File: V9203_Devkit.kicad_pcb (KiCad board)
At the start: 2 copper layers, 50 x 50 mm, 101 parts, among them J1 RJ45, J10 GS3, J2 CONN_01X16, J3 CONN_01X12, J4 Screw_Terminal_1x04, J5 GROVE-CONNECTOR-SMD-90D(4+2P-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, J6 CONN_01X09, J7 GS3, J8 GS3, J9 CONN_01X06, U1 V9203, U2 ROF-78E, Y1 Crystal_GND24

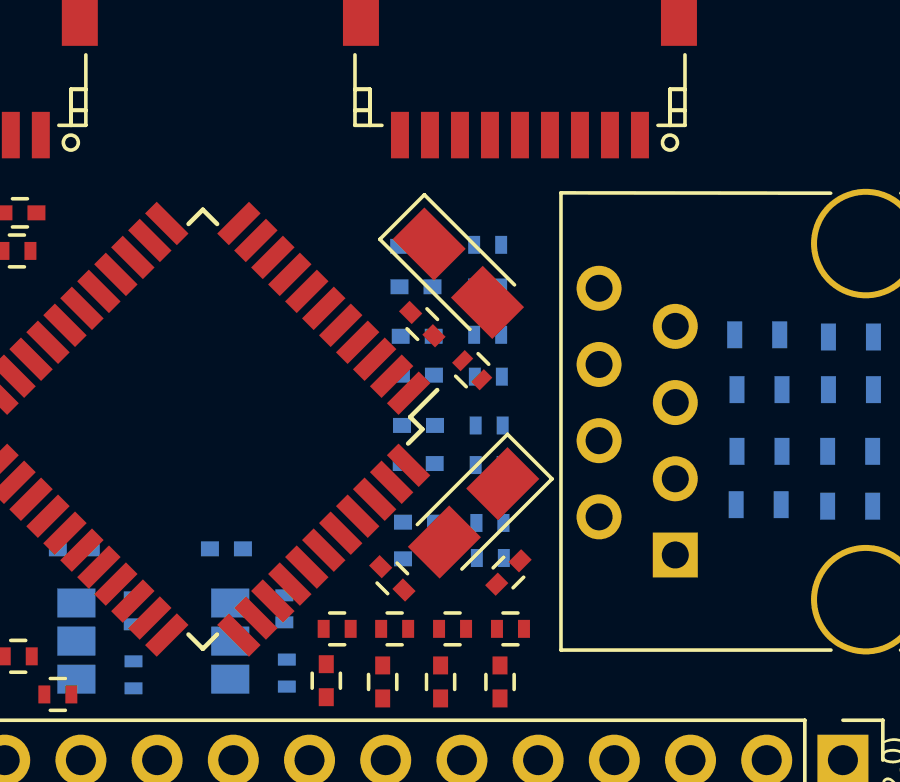
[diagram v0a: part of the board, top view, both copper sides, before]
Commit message: Set up for Freeroute
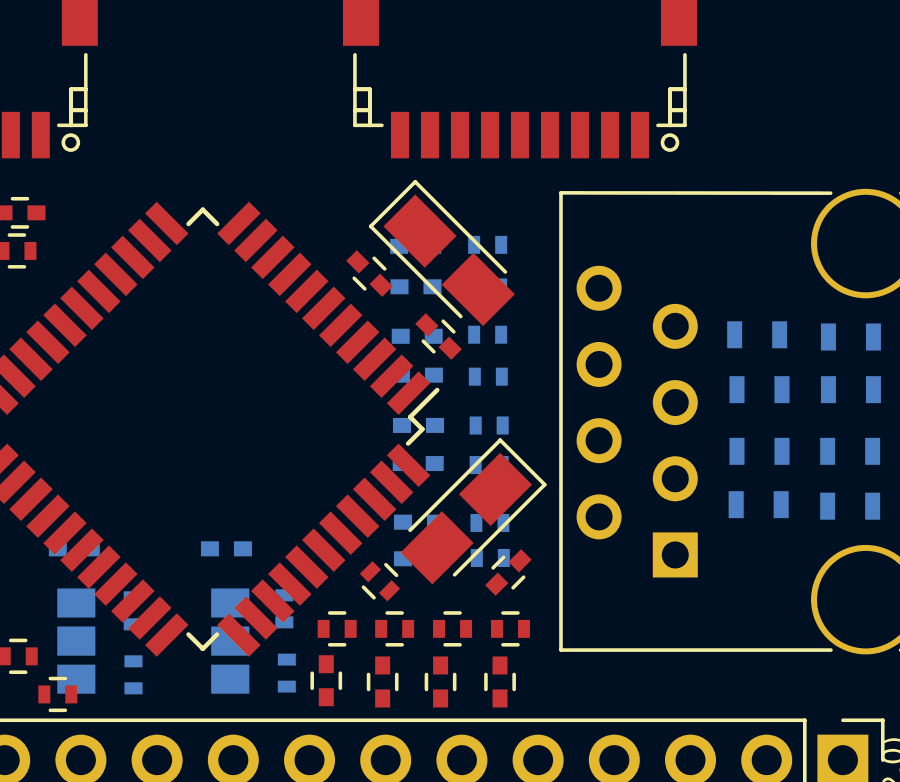
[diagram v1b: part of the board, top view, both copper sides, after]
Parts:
- moved C15 8.21 mm to (140.5, 52.4), turned to 135 degrees
- moved R33 7.68 mm to (138.5, 60.6), turned to 315 degrees
- moved C27 2.44 mm to (138.2, 50.3)
- moved C13 0.53 mm to (140.8, 49.9)
- moved C14 0.31 mm to (141.4, 58.5)
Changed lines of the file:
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@@
   )
   (module Capacitors_SMD:C_0402 (layer F.Cu)
-    (at 139.922629 51.987155 315)
+    (at 138.16212 50.302846 315)
     (descr "Capacitor SMD 0402, reflow soldering, AVX (see smccp.pdf)")
     (tags "capacitor 0402")
@@
   )
   (module Resistors_SMD:R_0402 (layer F.Cu)
-    (at 141.585631 53.524553 135)
+    (at 138.512231 60.558957 315)
     (descr "Resistor SMD 0402, reflow soldering, Vishay (see dcrcw.pdf)")
     (tags "resistor 0402")
     (attr smd)
-    (fp_text reference R33 (at 0 -1.35 135) (layer F.SilkS)
-      (effects (font (size 0.001 0.001) (thickness 0.00025)))
-    )
-    (fp_text value R (at 0 1.45 135) (layer F.Fab)
+    (fp_text reference R33 (at 0 -1.35 315) (layer F.SilkS)
+      (effects (font (size 0.001 0.001) (thickness 0.00025)))
+    )
+    (fp_text value R (at 0 1.45 315) (layer F.Fab)
       (effects (font (size 1 1) (thickness 0.15)))
     )
@@
     (fp_line (start 0.5 0.25) (end -0.5 0.25) (layer F.Fab) (width 0.1))
     (fp_line (start -0.5 0.25) (end -0.5 -0.25) (layer F.Fab) (width 0.1))
-    (fp_text user %R (at 0 -1.35 135) (layer F.Fab)
-      (effects (font (size 1 1) (thickness 0.15)))
-    )
-    (pad 2 smd rect (at 0.45 0 135) (size 0.4 0.6) (layers F.Cu F.Paste F.Mask)
+    (fp_text user %R (at 0 -1.35 315) (layer F.Fab)
+      (effects (font (size 1 1) (thickness 0.15)))
+    )
+    (pad 2 smd rect (at 0.45 0 315) (size 0.4 0.6) (layers F.Cu F.Paste F.Mask)
       (net 53 +3V3))
-    (pad 1 smd rect (at -0.45 0 135) (size 0.4 0.6) (layers F.Cu F.Paste F.Mask)
+    (pad 1 smd rect (at -0.45 0 315) (size 0.4 0.6) (layers F.Cu F.Paste F.Mask)
       (net 86 "Net-(R33-Pad1)"))
     (model ${KISYS3DMOD}/Resistors_SMD.3dshapes/R_0402.wrl
@@
   )
   (module Capacitors_SMD:C_0402 (layer F.Cu)
-    (at 138.92412 60.462846 315)
+    (at 140.463938 52.401464 135)
     (descr "Capacitor SMD 0402, reflow soldering, AVX (see smccp.pdf)")
     (tags "capacitor 0402")
     (attr smd)
-    (fp_text reference C15 (at 0 -1.27 315) (layer F.SilkS)
-      (effects (font (size 0.001 0.001) (thickness 0.00025)))
-    )
-    (fp_text value C (at 0 1.27 315) (layer F.Fab)
+    (fp_text reference C15 (at 0 -1.27 135) (layer F.SilkS)
+      (effects (font (size 0.001 0.001) (thickness 0.00025)))
+    )
+    (fp_text value C (at 0 1.27 135) (layer F.Fab)
       (effects (font (size 1 1) (thickness 0.15)))
     )
@@
     (fp_line (start 0.5 0.25) (end -0.5 0.25) (layer F.Fab) (width 0.1))
     (fp_line (start -0.5 0.25) (end -0.5 -0.25) (layer F.Fab) (width 0.1))
-    (fp_text user %R (at 0 -1.27 315) (layer F.Fab)
-      (effects (font (size 1 1) (thickness 0.15)))
-    )
-    (pad 2 smd rect (at 0.55 0 315) (size 0.6 0.5) (layers F.Cu F.Paste F.Mask)
+    (fp_text user %R (at 0 -1.27 135) (layer F.Fab)
+      (effects (font (size 1 1) (thickness 0.15)))
+    )
+    (pad 2 smd rect (at 0.55 0 135) (size 0.6 0.5) (layers F.Cu F.Paste F.Mask)
       (net 33 "Net-(C14-Pad2)"))
-    (pad 1 smd rect (at -0.55 0 315) (size 0.6 0.5) (layers F.Cu F.Paste F.Mask)
+    (pad 1 smd rect (at -0.55 0 135) (size 0.6 0.5) (layers F.Cu F.Paste F.Mask)
       (net 35 "Net-(C13-Pad1)"))
     (model Capacitors_SMD.3dshapes/C_0402.wrl
@@
   )
   (module Capacitors_Tantalum_SMD:CP_Tantalum_Case-A_EIA-3216-18_Reflow (layer F.Cu)
-    (at 141.631501 58.279283 225)
+    (at 141.388757 58.471227 225)
     (descr "Tantalum capacitor, Case A, EIA 3216-18, 3.2x1.6x1.6mm, Reflow soldering footprint")
     (tags "capacitor tantalum smd")
@@
   )
   (module Capacitors_Tantalum_SMD:CP_Tantalum_Case-A_EIA-3216-18_Reflow (layer F.Cu)
-    (at 141.123501 50.292427 315)
+    (at 140.818701 49.860627 315)
     (descr "Tantalum capacitor, Case A, EIA 3216-18, 3.2x1.6x1.6mm, Reflow soldering footprint")
     (tags "capacitor tantalum smd")

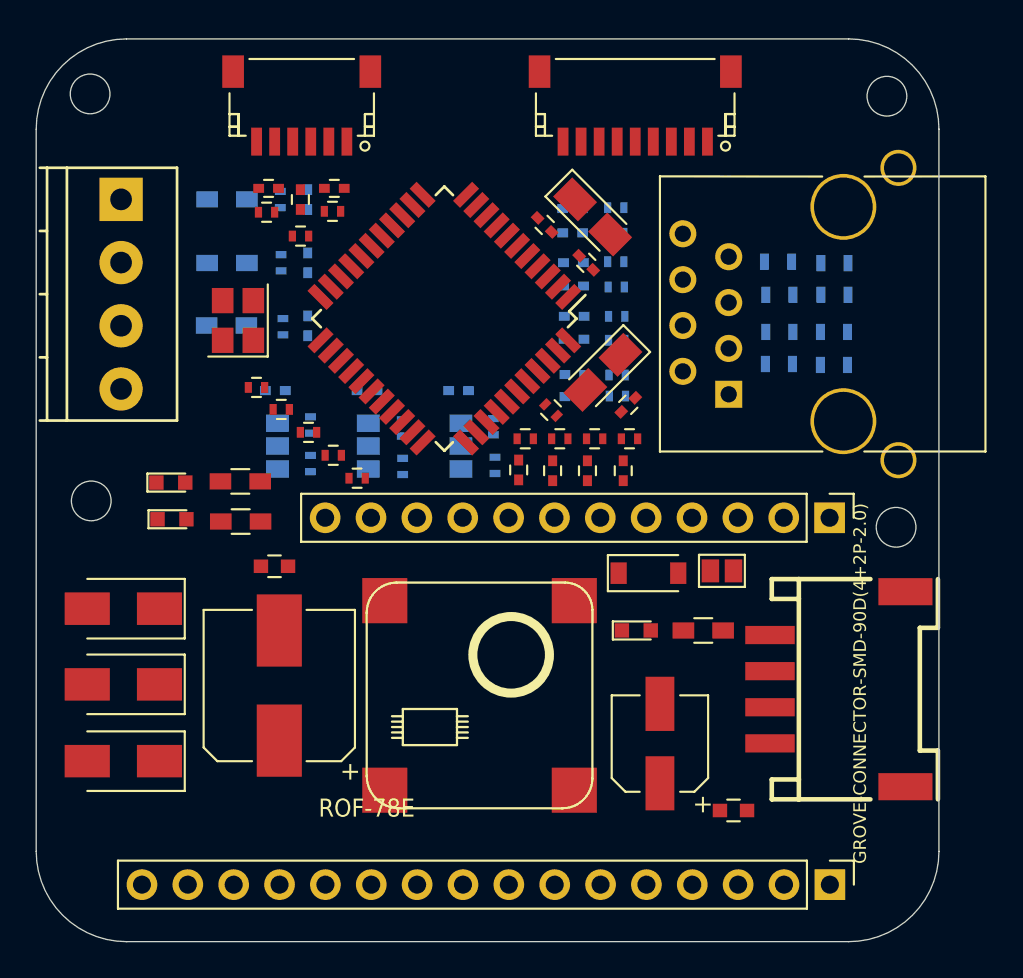
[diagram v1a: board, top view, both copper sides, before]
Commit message: Freeroute run
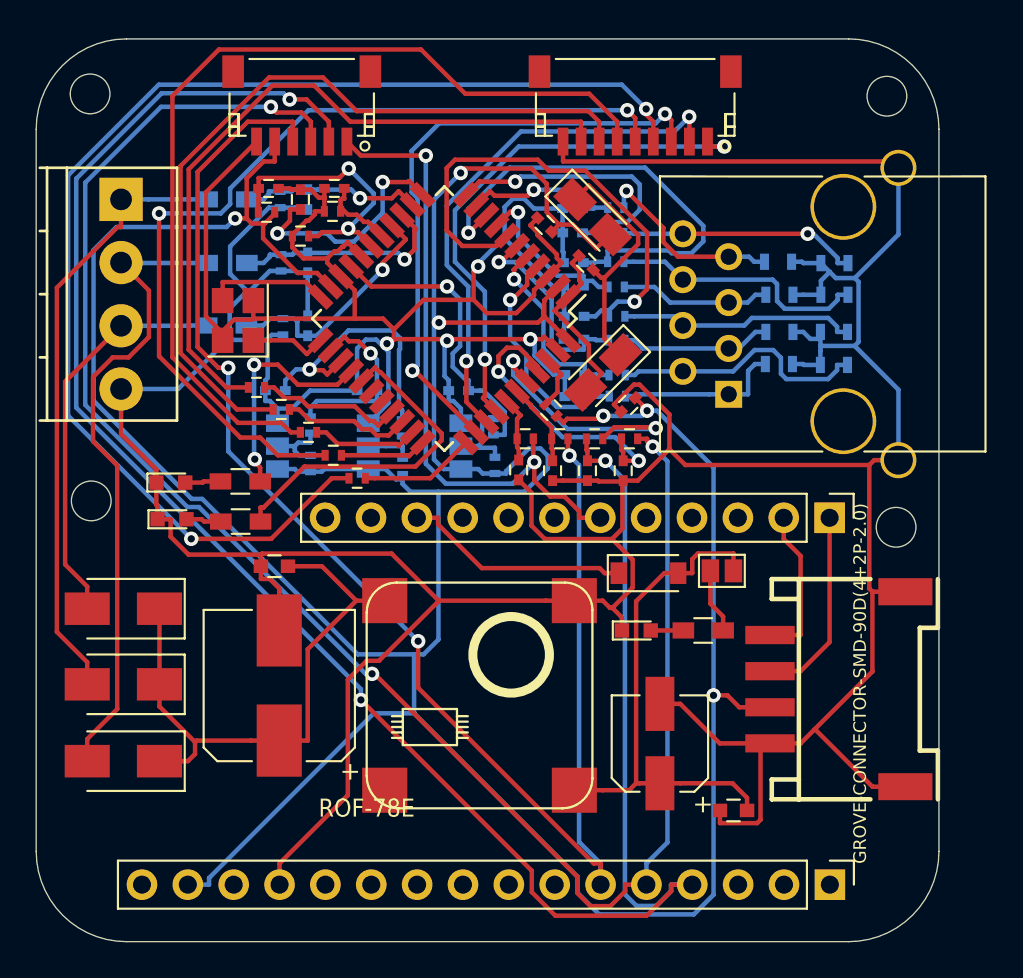
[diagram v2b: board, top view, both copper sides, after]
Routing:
- net GND: track 0.00 -> 339.4 mm, vias 0 -> 4
- net +3V3: track 0.00 -> 207.8 mm, vias 0 -> 6
- net MISO: track 0.00 -> 109.5 mm, vias 0 -> 3
- net MOSI: track 0.00 -> 98.0 mm, vias 0 -> 3
- net SCK: track 0.00 -> 82.2 mm, vias 0 -> 3
- net Net-(J6-Pad4): track 0.00 -> 69.7 mm, vias 0 -> 2
- net Net-(J6-Pad6): track 0.00 -> 51.7 mm
- net Net-(J6-Pad5): track 0.00 -> 50.1 mm, vias 0 -> 2
- net Net-(J6-Pad7): track 0.00 -> 44.1 mm
- net Net-(J6-Pad8): track 0.00 -> 39.7 mm
- net UB: track 0.00 -> 36.1 mm
- net CS: track 0.00 -> 35.8 mm, vias 0 -> 2
- net Net-(J6-Pad3): track 0.00 -> 33.9 mm, vias 0 -> 2
- net UA: track 0.00 -> 33.9 mm
- net Net-(C1-Pad1): track 0.00 -> 32.3 mm
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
